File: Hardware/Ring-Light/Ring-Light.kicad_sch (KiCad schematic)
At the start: 12 parts, among them U1 74HC595, U2 74HC595, U5 74HC595, U6 74HC595

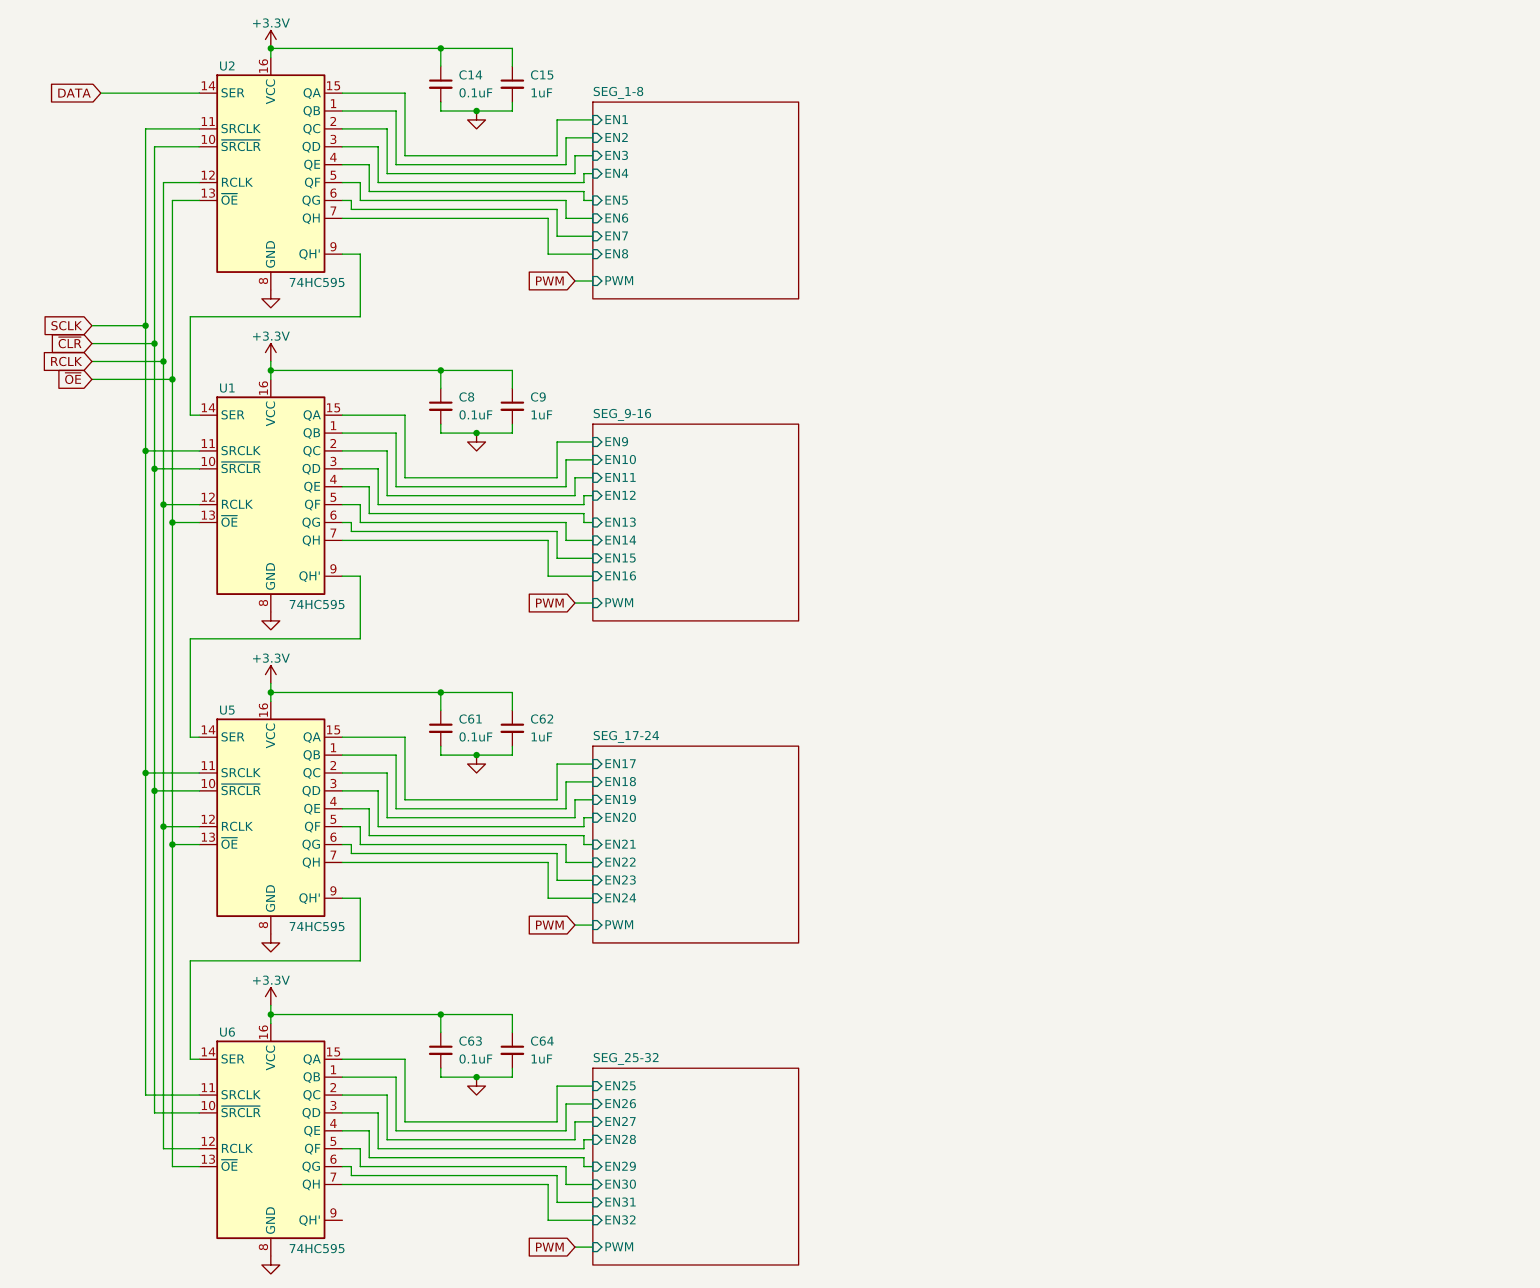
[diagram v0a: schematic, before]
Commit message: m
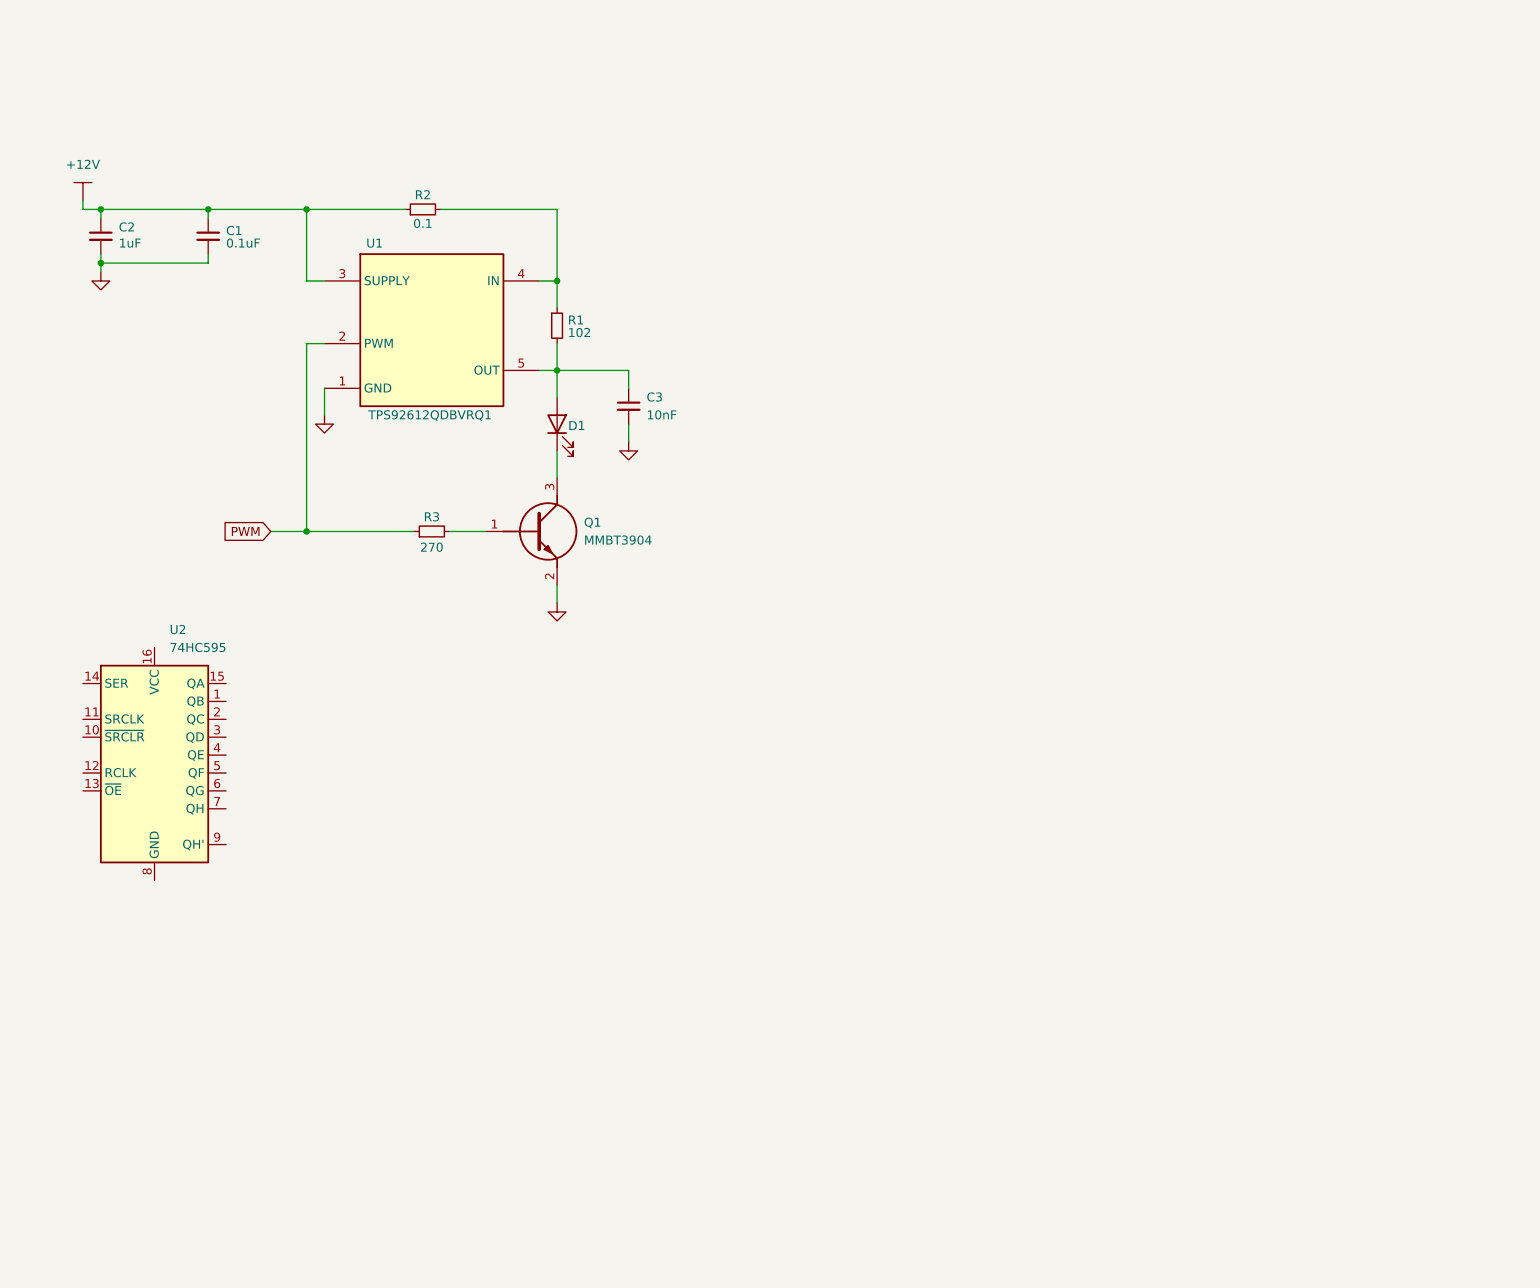
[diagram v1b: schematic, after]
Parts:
- removed C14, C61, C63, C8: 0.1uF, symbol Device:C_Small
- removed C15, C62, C64, C9: 1uF, symbol Device:C_Small
- removed U1, U5, U6: 74HC595, symbol 74xx:74HC595
- added C1: 0.1uF, Capacitor_SMD:C_0603_1608Metric, symbol Device:C_Small
- added C2: 1uF, Capacitor_SMD:C_0805_2012Metric, symbol Device:C_Small
- added C3: 10nF, Capacitor_SMD:C_0603_1608Metric, symbol Device:C_Small
- added D1: LED, Library:GWJTLRS1EMLVL5XX531, symbol Library:LED
- added Q1: MMBT3904, Library:SOT95P240X120-3N, symbol Library:MMBT3904
- added R1: 102, Resistor_SMD:R_1210_3225Metric, symbol Device:R_Small
- added R2: 0.1, Resistor_SMD:R_0805_2012Metric, symbol Device:R_Small
- added R3: 270, Resistor_SMD:R_0603_1608Metric, symbol Device:R_Small
- added U1: TPS92612QDBVRQ1, Library:SOT95P280X145-5N, symbol Library:TPS92612QDBVRQ1
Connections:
- net GND: now also C1.2, C2.2, C3.2, Q1.2 (E), U1.1 (GND); no longer U2.8 (GND)
- net PWM: now also R3.1, U1.2 (PWM)
- net +3.3V: no longer names the net of U2.16 (VCC)
- net DATA: no longer names the net of U2.14 (SER)
- net RCLK: no longer names the net of U2.12 (RCLK)
- net SCLK: no longer names the net of U2.11 (SRCLK)
- net SEG_1-8/EN1: no longer names the net of U2.15 (QA)
- net SEG_1-8/EN2: no longer names the net of U2.1 (QB)
- net SEG_1-8/EN3: no longer names the net of U2.2 (QC)
- net SEG_1-8/EN4: no longer names the net of U2.3 (QD)
- net SEG_1-8/EN5: no longer names the net of U2.4 (QE)
- net SEG_1-8/EN6: no longer names the net of U2.5 (QF)
- net SEG_1-8/EN7: no longer names the net of U2.6 (QG)
- net SEG_1-8/EN8: no longer names the net of U2.7 (QH)
- net ~{CLR}: no longer names the net of U2.10 (~{SRCLR})
- net ~{OE}: no longer names the net of U2.13 (~{OE})
- new net: Q1.1 (B), R3.2
- new net: C3.1, D1.3 (A), D1.4 (A), R1.2, U1.5 (OUT)
- new net: R1.1, R2.2, U1.4 (IN)
- new net: D1.1 (K), D1.2 (K), Q1.3 (C)
- new net +12V: C1.1, C2.1, R2.1, U1.3 (SUPPLY)
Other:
- removed sheet SEG_1-8
- removed sheet SEG_17-24
- removed sheet SEG_25-32
- removed sheet SEG_9-16

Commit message: m
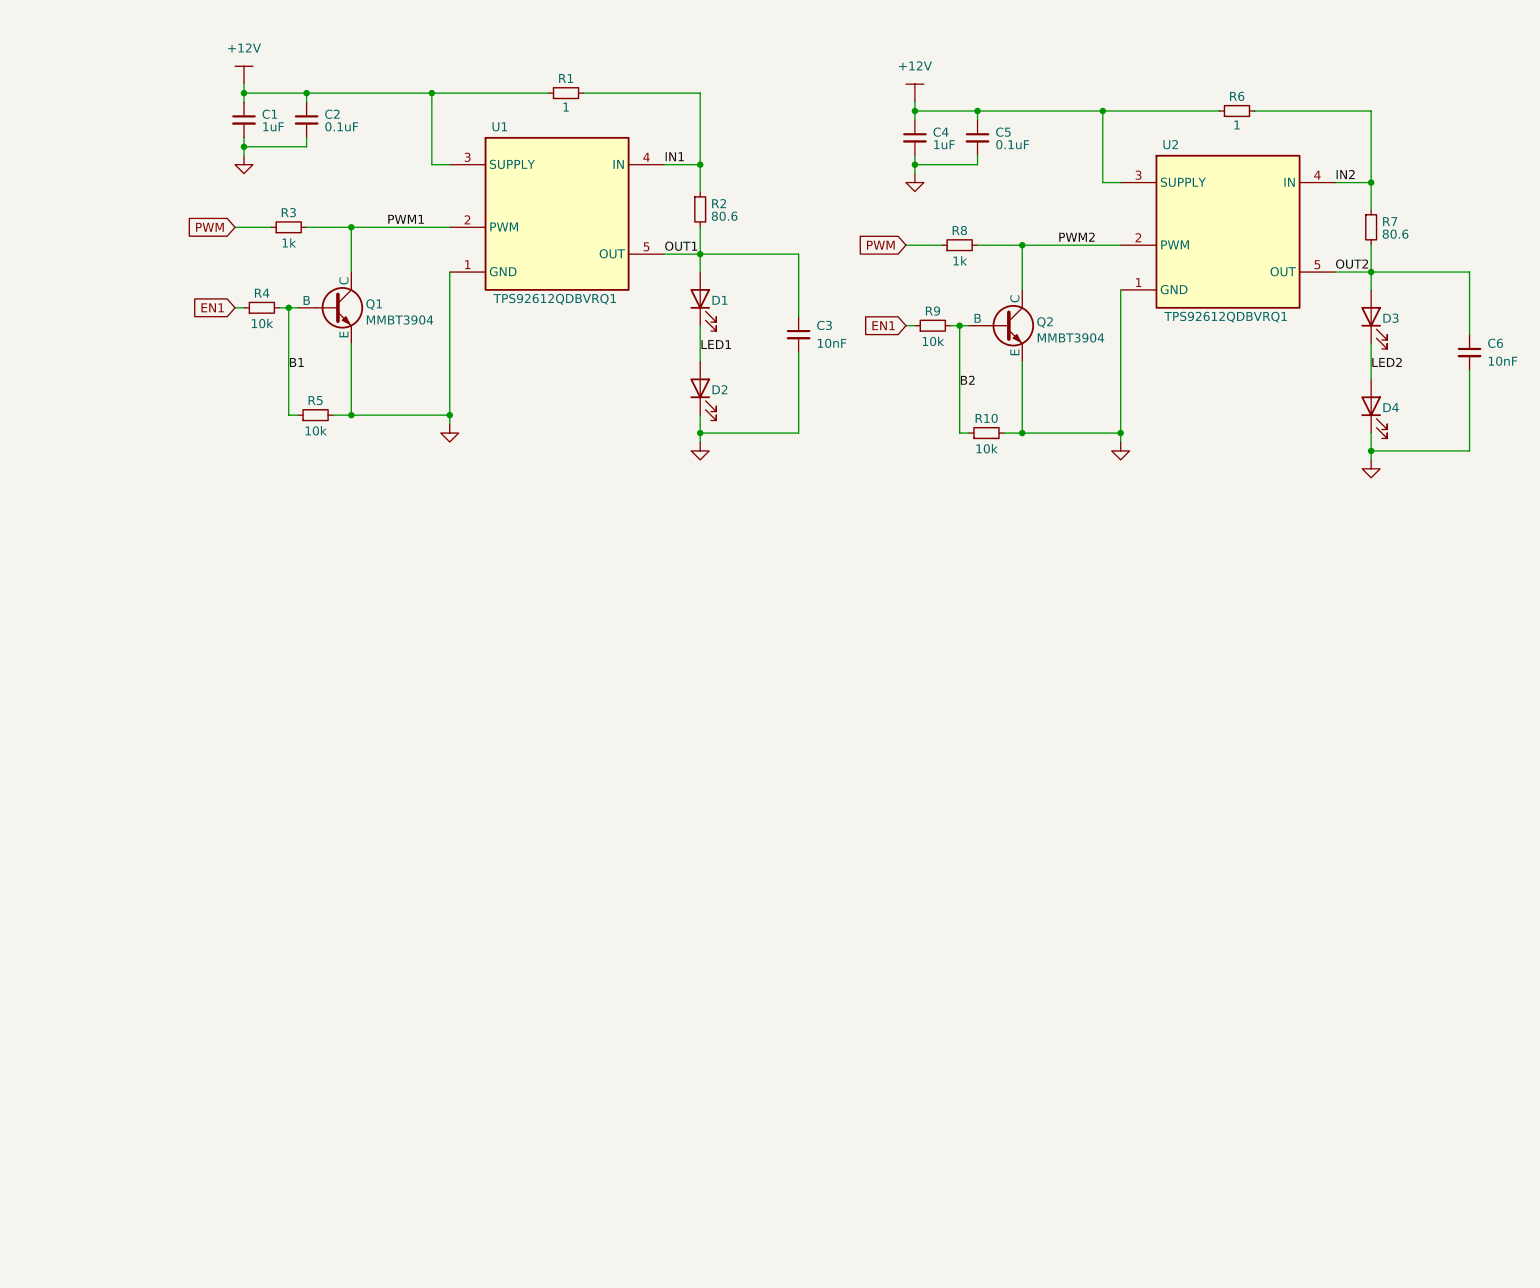
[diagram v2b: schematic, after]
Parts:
- removed Q1: MMBT3904, Library:SOT95P240X120-3N, symbol Library:MMBT3904
- removed U2: 74HC595, symbol 74xx:74HC595
- added C4: 1uF, Capacitor_SMD:C_0805_2012Metric, symbol Device:C_Small
- added C5: 0.1uF, Capacitor_SMD:C_0603_1608Metric, symbol Device:C_Small
- added C6: 10nF, Capacitor_SMD:C_0402_1005Metric, symbol Device:C_Small
- added D2, D3, D4: LED, Library:GWJTLRS1EMLVL5XX531, symbol Library:LED
- added Q1, Q2: MMBT3904, Package_TO_SOT_SMD:SOT-416, symbol Library:MMBT39042-2
- added R10, R5, R9: 10k, Resistor_SMD:R_0402_1005Metric, symbol Device:R_Small
- added R3, R8: 1k, Resistor_SMD:R_0402_1005Metric, symbol Device:R_Small
- added R6: 1, Resistor_SMD:R_0402_1005Metric, symbol Device:R_Small
- added R7: 80.6, Resistor_SMD:R_1210_3225Metric, symbol Device:R_Small
- added U2: TPS92612QDBVRQ1, Library:SOT95P280X145-5N, symbol Library:TPS92612QDBVRQ1
- C3: footprint Capacitor_SMD:C_0603_1608Metric -> Capacitor_SMD:C_0402_1005Metric
- R1: renamed from R2; value 0.1 -> 1; footprint Resistor_SMD:R_0805_2012Metric -> Resistor_SMD:R_0402_1005Metric
- R2: renamed from R1; value 102 -> 80.6
- R4: renamed from R3; value 270 -> 10k; footprint Resistor_SMD:R_0603_1608Metric -> Resistor_SMD:R_0402_1005Metric
- renumbered C2 to C1, C1 to C2
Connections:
- net +12V: now also C4.1, C5.1, R6.1, U2.3 (SUPPLY)
- net GND: now also C4.2, C5.2, C6.2, D2.1 (K), D2.2 (K), D4.1 (K), D4.2 (K), Q1.2 (E), Q2.2 (E), R10.2, R5.2, U2.1 (GND)
- net PWM: now also R3.1, R8.1; no longer R4.1, U1.2 (PWM)
- net B1: now reaches R4.2
- net B1: now also Q1.1 (B), R5.1
- net OUT1: now reaches C3.1, D1.3 (A), D1.4 (A), R2.2, U1.5 (OUT)
- net IN1: now reaches R1.2, R2.1, U1.4 (IN)
- net LED1: now reaches D1.1 (K), D1.2 (K)
- net LED1: now also D2.3 (A), D2.4 (A)
- new net B2: Q2.1 (B), R10.1, R9.2
- new net EN1: R4.1, R9.1
- new net IN2: R6.2, R7.1, U2.4 (IN)
- new net LED2: D3.1 (K), D3.2 (K), D4.3 (A), D4.4 (A)
- new net OUT2: C6.1, D3.3 (A), D3.4 (A), R7.2, U2.5 (OUT)
- new net PWM1: Q1.3 (C), R3.2, U1.2 (PWM)
- new net PWM2: Q2.3 (C), R8.2, U2.2 (PWM)
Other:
- moved on the sheet: C1, C2, C3, D1, R1, R2, R4, U1
